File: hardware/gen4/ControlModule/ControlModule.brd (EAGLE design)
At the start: 96.7 x 75.3 mm, 40 parts, among them IC1 XMEGA16A4A

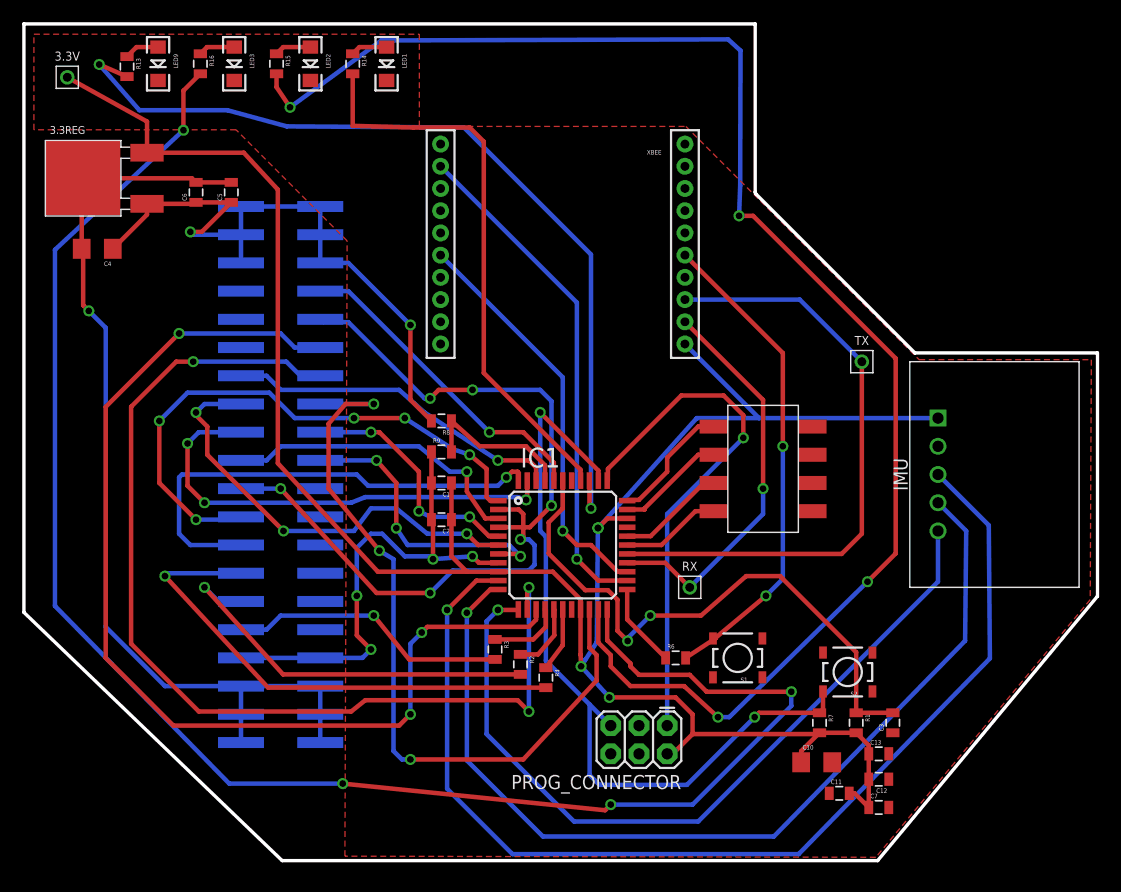
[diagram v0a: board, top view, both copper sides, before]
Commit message: almost done with shrinking comms board but computer is at 2 percent and I dont have a charger :/
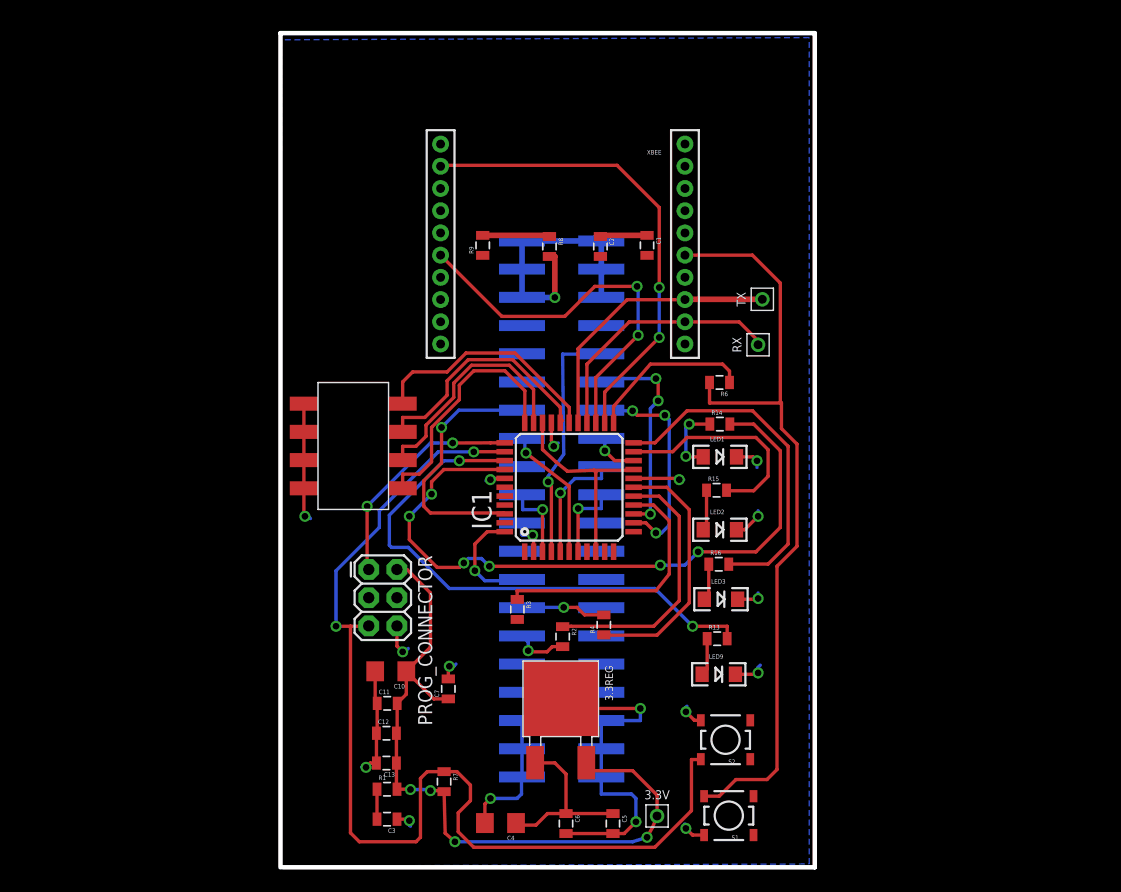
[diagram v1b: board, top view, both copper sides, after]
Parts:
- removed IMU: MPU6050IMUMPU, gen3:MPU-6050IMU
- moved 3.3V 85.1 mm to (57.0, 4.02)
- moved LED9 74.6 mm to (62.6, 16.8), turned to 0 degrees
- moved R13 74.0 mm to (62.4, 20.0), turned to 0 degrees
- moved C5 66.4 mm to (53.0, 3.34), turned to 270 degrees
- moved C6 65.9 mm to (48.8, 3.34), turned to 270 degrees
- moved LED3 65.2 mm to (62.8, 23.5), turned to 0 degrees
- moved R16 64.9 mm to (62.6, 26.7), turned to 0 degrees
- moved 3.3REG 63.6 mm to (48.3, 14.6), turned to 270 degrees
- moved C4 63.2 mm to (42.9, 3.38)
- moved LED2 55.8 mm to (62.7, 29.8), turned to 0 degrees
- moved R15 55.2 mm to (62.4, 33.3), turned to 0 degrees
- moved LED1 46.4 mm to (62.7, 36.4), turned to 0 degrees
- moved C3 46.4 mm to (32.7, 3.73), turned to 180 degrees
- moved R14 46.3 mm to (62.7, 39.3), turned to 0 degrees
- moved C12 44.5 mm to (32.6, 11.5), turned to 0 degrees
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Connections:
- net 3.3V: no longer IMU.VCC
- net GND: no longer IMU.GND
- net INT: no longer IMU.INT
- net SCL: no longer IMU.SCL
- net SDA: no longer IMU.SDA
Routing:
- net RLED2: track 153.3 -> 31.3 mm, vias 4 -> 0
- net GLED2: track 137.3 -> 19.8 mm, vias 4 -> 0
- net 3.3V: track 201.4 -> 88.9 mm
- net SDA: track 99.0 -> 0.00 mm, vias 1 -> 0
- net SCL: track 85.6 -> 0.00 mm, vias 1 -> 0
- net KICK_ENABLE: track 95.0 -> 19.1 mm
- net CHIP_ENABLE: track 92.9 -> 19.9 mm
- net INT: track 70.9 -> 0.00 mm, vias 1 -> 0
- net KICK_REF: track 69.9 -> 4.20 mm, vias 3 -> 1
- net N$1: track 53.7 -> 2.70 mm, vias 2 -> 0
- net SS_3: track 51.0 -> 0.00 mm, vias 5 -> 0
- net DRIB: track 42.1 -> 0.00 mm, vias 3 -> 0
- net N$8: track 45.6 -> 7.66 mm
- net SS_2: track 39.7 -> 3.57 mm, vias 3 -> 1
- net 12VGND: track 86.5 -> 50.5 mm, vias 1 -> 3
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- added copper zone on layer 16, net GND
- removed copper zone on layer 1, net GND
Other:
- board size 96.7 x 75.3 mm -> 48.1 x 75.1 mm
